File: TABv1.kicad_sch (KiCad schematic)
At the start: 40 parts, among them J10 Conn_02x03_Odd_Even, J5 Conn_02x08_Odd_Even, J6 Conn_02x08_Odd_Even, J9 Conn_02x03_Odd_Even, Q3 DMN2040U, SW2 RESET, U1 RP2350B-QFN80, Y1 12MHz

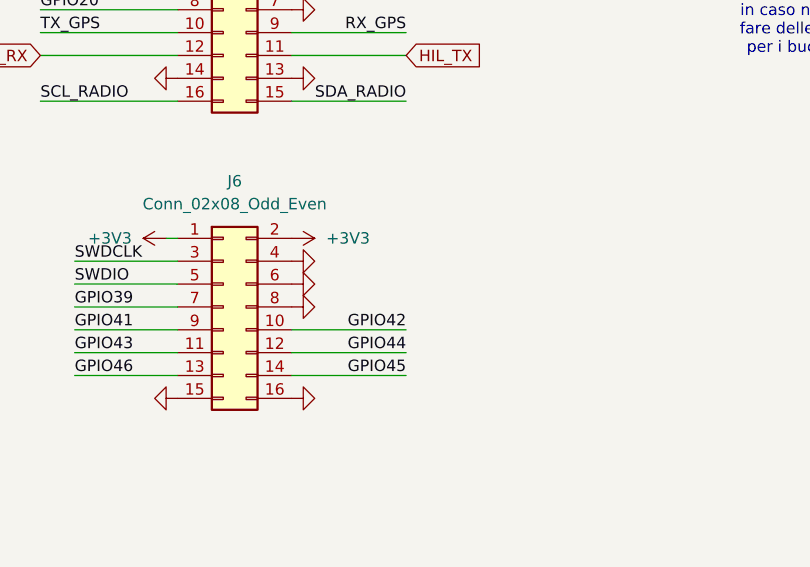
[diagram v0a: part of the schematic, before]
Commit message: small fixes, started working on the backpack
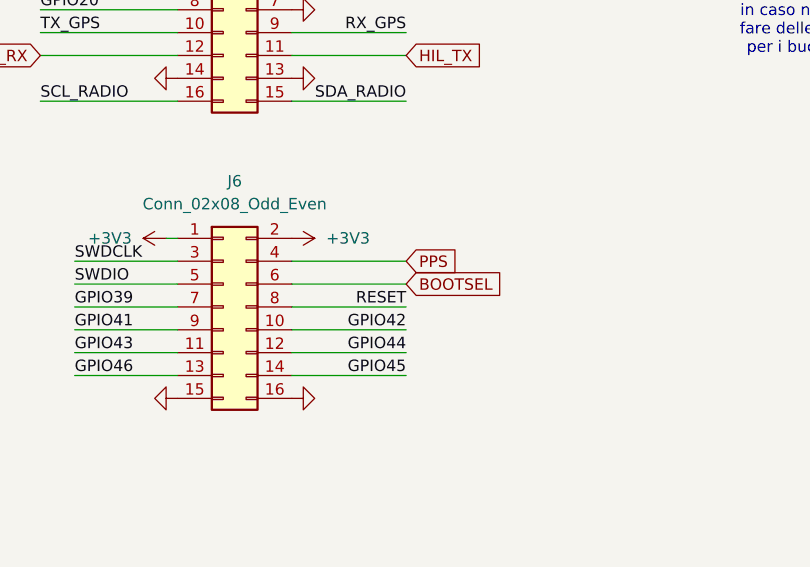
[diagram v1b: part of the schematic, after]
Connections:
- net GND: no longer J6.4 (Pin_4), J6.6 (Pin_6), J6.8 (Pin_8)
- net PPS: now also J6.4 (Pin_4)
- net RESET: now also J6.8 (Pin_8)
- new net BOOTSEL: J6.6 (Pin_6)
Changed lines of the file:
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@@
 		)
 	)
+	(wire
+		(pts
+			(xy 267.97 115.57) (xy 255.27 115.57)
+		)
+		(stroke
+			(width 0)
+			(type default)
+		)
+	)
 	(polyline
 		(pts
@@
 	(wire
 		(pts
+			(xy 267.97 110.49) (xy 255.27 110.49)
+		)
+		(stroke
+			(width 0)
+			(type default)
+		)
+	)
+	(wire
+		(pts
 			(xy 129.54 106.68) (xy 165.1 106.68)
 		)
@@
 	(wire
 		(pts
+			(xy 267.97 113.03) (xy 255.27 113.03)
+		)
+		(stroke
+			(width 0)
+			(type default)
+		)
+	)
+	(wire
+		(pts
 			(xy 58.42 241.3) (xy 60.96 241.3)
 		)
@@
 		)
 	)
+	(label "RESET"
+		(at 267.97 115.57 180)
+		(effects
+			(font
+				(size 1.27 1.27)
+			)
+			(justify right bottom)
+		)
+	)
 	(label "SD0"
 		(at 39.37 77.47 0)
@@
 		)
 	)
+	(global_label "BOOTSEL"
+		(shape input)
+		(at 267.97 113.03 0)
+		(fields_autoplaced yes)
+		(effects
+			(font
+				(size 1.27 1.27)
+			)
+			(justify left)
+		)
+		(property "Intersheetrefs" "${INTERSHEET_REFS}"
+			(at 279.2404 113.03 0)
+			(effects
+				(font
+					(size 1.27 1.27)
+				)
+				(justify left)
+				(hide yes)
+			)
+		)
+	)
 	(global_label "PPS"
 		(shape input)
@@
 		)
 	)
+	(global_label "PPS"
+		(shape input)
+		(at 267.97 110.49 0)
+		(fields_autoplaced yes)
+		(effects
+			(font
+				(size 1.27 1.27)
+			)
+			(justify left)
+		)
+		(property "Intersheetrefs" "${INTERSHEET_REFS}"
+			(at 274.7047 110.49 0)
+			(effects
+				(font
+					(size 1.27 1.27)
+				)
+				(justify left)
+				(hide yes)
+			)
+		)
+	)
 	(global_label "HIL_RX"
 		(shape input)
@@
 	(symbol
 		(lib_id "power:GND")
-		(at 255.27 110.49 90)
-		(unit 1)
-		(exclude_from_sim no)
-		(in_bom yes)
-		(on_board yes)
-		(dnp no)
-		(fields_autoplaced yes)
-		(property "Reference" "#PWR0143"
-			(at 261.62 110.49 0)
-			(effects
-				(font
-					(size 1.27 1.27)
-				)
-				(hide yes)
-			)
-		)
-		(property "Value" "GND"
-			(at 259.08 110.4901 90)
-			(effects
-				(font
-					(size 1.27 1.27)
-				)
-				(justify right)
-				(hide yes)
-			)
-		)
-		(property "Footprint" ""
-			(at 255.27 110.49 0)
-			(effects
-				(font
-					(size 1.27 1.27)
-				)
-				(hide yes)
-			)
-		)
-		(property "Datasheet" ""
-			(at 255.27 110.49 0)
-			(effects
-				(font
-					(size 1.27 1.27)
-				)
-				(hide yes)
-			)
-		)
-		(property "Description" "Power symbol creates a global label with name \"GND\" , ground"
-			(at 255.27 110.49 0)
-			(effects
-				(font
-					(size 1.27 1.27)
-				)
-				(hide yes)
-			)
-		)
-		(pin "1"
-		)
-		(instances
-			(project "TABv1"
-				(path "/105f6e80-8e20-4d56-8eb3-6fa826818670"
-					(reference "#PWR0143")
-					(unit 1)
-				)
-			)
-		)
-	)
-	(symbol
-		(lib_id "power:GND")
 		(at 266.7 242.57 90)
 		(unit 1)
@@
 	(symbol
 		(lib_id "power:GND")
-		(at 255.27 113.03 90)
-		(unit 1)
-		(exclude_from_sim no)
-		(in_bom yes)
-		(on_board yes)
-		(dnp no)
-		(fields_autoplaced yes)
-		(property "Reference" "#PWR0142"
-			(at 261.62 113.03 0)
-			(effects
-				(font
-					(size 1.27 1.27)
-				)
-				(hide yes)
-			)
-		)
-		(property "Value" "GND"
-			(at 259.08 113.0301 90)
-			(effects
-				(font
-					(size 1.27 1.27)
-				)
-				(justify right)
-				(hide yes)
-			)
-		)
-		(property "Footprint" ""
-			(at 255.27 113.03 0)
-			(effects
-				(font
-					(size 1.27 1.27)
-				)
-				(hide yes)
-			)
-		)
-		(property "Datasheet" ""
-			(at 255.27 113.03 0)
-			(effects
-				(font
-					(size 1.27 1.27)
-				)
-				(hide yes)
-			)
-		)
-		(property "Description" "Power symbol creates a global label with name \"GND\" , ground"
-			(at 255.27 113.03 0)
-			(effects
-				(font
-					(size 1.27 1.27)
-				)
-				(hide yes)
-			)
-		)
-		(pin "1"
-		)
-		(instances
-			(project "TABv1"
-				(path "/105f6e80-8e20-4d56-8eb3-6fa826818670"
-					(reference "#PWR0142")
-					(unit 1)
-				)
-			)
-		)
-	)
-	(symbol
-		(lib_id "power:GND")
 		(at 255.27 82.55 90)
 		(unit 1)
@@
 					(unit 1)
 				)
-			)
-		)
-	)
-	(symbol
-		(lib_id "power:GND")
-		(at 255.27 115.57 90)
-		(unit 1)
-		(exclude_from_sim no)
-		(in_bom yes)
-		(on_board yes)
-		(dnp no)
-		(fields_autoplaced yes)
-		(property "Reference" "#PWR0141"
-			(at 261.62 115.57 0)
-			(effects
-				(font
-					(size 1.27 1.27)
-				)
-				(hide yes)
-			)
-		)
-		(property "Value" "GND"
-			(at 259.08 115.5701 90)
-			(effects
-				(font
-					(size 1.27 1.27)
-				)
-				(justify right)
-				(hide yes)
-			)
-		)
-		(property "Footprint" ""
-			(at 255.27 115.57 0)
-			(effects
-				(font
-					(size 1.27 1.27)
-				)
-				(hide yes)
-			)
-		)
-		(property "Datasheet" ""
-			(at 255.27 115.57 0)
-			(effects
-				(font
-					(size 1.27 1.27)
-				)
-				(hide yes)
-			)
-		)
-		(property "Description" "Power symbol creates a global label with name \"GND\" , ground"
-			(at 255.27 115.57 0)
-			(effects
-				(font
-					(size 1.27 1.27)
-				)
-				(hide yes)
-			)
-		)
-		(pin "1"
-		)
-		(instances
-			(project "TABv1"
-				(path "/105f6e80-8e20-4d56-8eb3-6fa826818670"
-					(reference "#PWR0141")
-					(unit 1)
-				)
